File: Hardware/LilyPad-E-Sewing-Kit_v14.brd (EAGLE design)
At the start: 133.1 x 52.3 mm, 91 parts

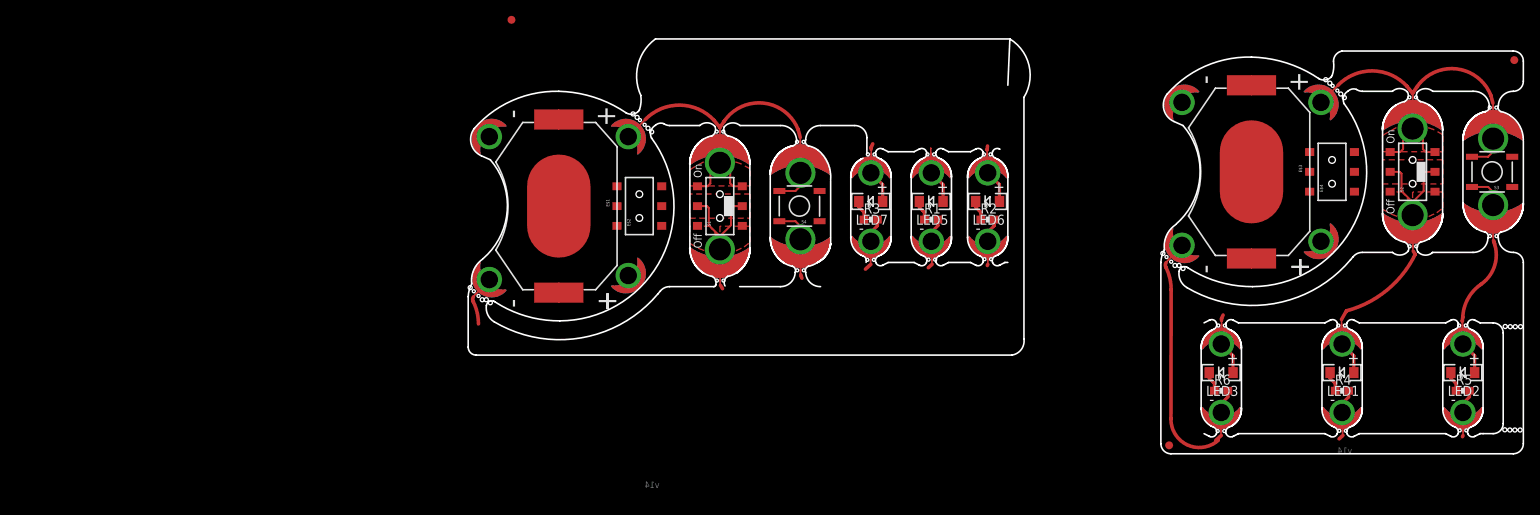
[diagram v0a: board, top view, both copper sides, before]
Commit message: Updated board file
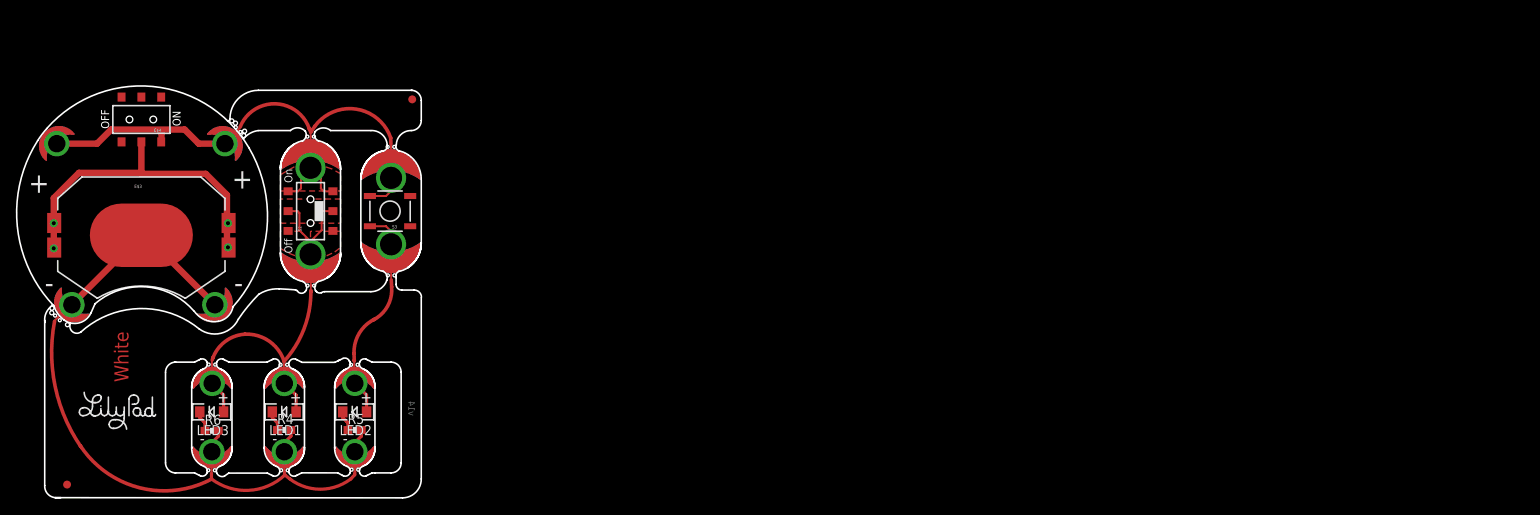
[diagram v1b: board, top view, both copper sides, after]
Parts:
- removed BUTTON-1, BUTTONS1, SLIDEOFF1, SLIDEON1: SEWTAP8, LilyPad-Wearables:PETAL-MEDIUM-2SIDE
- removed E$1: (no value), SparkFun-Electromechanical:BATTCON_20MM_4LEGS
- removed E$2: (no value), SparkFun-Electromechanical:AYZ0202
- removed JP4, JP6: LOGO-SFESK, SparkFun-Aesthetics:SFE-LOGO-FLAME
- removed JP5: FIDUCIAL1X2, SparkFun:FIDUCIAL-1X2
- removed LED+5, LED+6, LED+7, LED-5, LED-6, LED-7, U$34, U$35, U$36, U$37: SEWTAP6, LilyPad-Wearables:PETAL-SMALL-2SIDE
- removed LED5, LED6, LED7: White, SparkFun-3-2-07:LED-1206
- removed LOGO10, LOGO11, LOGO14, LOGO8, LOGO9: LOGO-LPL, LilyPad-Wearables:LOGO-L
- removed R1, R2, R3: 100, SparkFun:0603-RES
- removed S1: AYZ0202, SparkFun:AYZ0202
- removed S4: (no value), SparkFun:TACTILE_SWITCH_SMD
- removed U$18, U$43: OSHW-LOGOS, SparkFun-Aesthetics:OSHW-LOGO-S
- removed U$22, U$23, U$24, U$27, U$28, U$29, U$30, U$31, U$32, U$33, U$39, U$41: MOUSE-BITE-12_HOLES, Testing:MOUST-BITE-1-(2_HOLES)
- removed U$38: LOGO-LPLP, LilyPad-Wearables:LOGO-LILYPAD
- added E$5: (no value), LilyPad-Wearables:LOGO-LILYPAD
- E$3: device SparkFun-Electromechanical:BATTCON_20MM_4LEGS -> SparkFun-Electromechanical:BATTCON_20MM_4LEGS_OVERPASTE
- R4, R5, R6: value 100 -> 180
- moved U$12 159.5 mm to (1.45, 44.7), turned to 223 degrees
- moved E$4 150.3 mm to (12.1, 47.8), turned to 180 degrees
- moved U$15 143.9 mm to (12.1, 37.0), turned to 0 degrees
- moved U$11 142.3 mm to (3.35, 24.4), turned to 317 degrees
- moved U$17 140.4 mm to (1.52, 22.7), turned to 45 degrees
- moved E$3 140.3 mm to (12.1, 33.1), turned to 0 degrees
- moved LED+2 139.9 mm to (39.0, 14.5)
- moved LED-2 139.9 mm to (39.0, 5.84)
- moved U$5 139.9 mm to (39.0, 3.58)
- moved LED2 139.9 mm to (39.0, 10.9)
- moved R5 139.9 mm to (39.0, 8.59)
- moved U$2 139.9 mm to (39.0, 16.8)
- moved LOGO5 139.8 mm to (39.1, 9.80)
- moved BUTTON-2 139.1 mm to (43.6, 40.1)
- moved BUTTONS2 139.1 mm to (43.6, 32.3)
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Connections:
- removed net BUTTON1: BUTTONS1.1, S4.2, U$31.P$1
- removed net N$1: LED5.C, R1.1
- removed net N$2: LED6.C, R2.1
- removed net N$3: LED7.C, R3.1
- removed net S$1: LED+7.1, LED7.A, U$22.P$1
- removed net S$10: LED+6.1, LED6.A, U$23.P$1
- removed net S$11: LED+5.1, LED5.A, U$24.P$1
- removed net S$3: LED-6.1, R2.2, U$28.P$1
- removed net S$4: LED-5.1, R1.2, U$29.P$1
- removed net S$9: U$34.1, U$36.1, U$41.P$1
- removed net SINK3: S1.4
- removed net SINK4: S1.1
- removed net SWITCH1: S1.2, S1.5, SLIDEOFF1.1, U$32.P$1
- removed net VCC1: BUTTON-1.1, S1.3, S1.6, S4.4, SLIDEON1.1, U$30.P$1, U$33.P$1, U$35.1, U$37.1, U$39.P$1
- new net S$16: LED+2.1, LED2.A
- new net S$25: U$2.P$1
- new net S$26: LED+1.1, LED1.A, U$3.P$1
- net BUTTON2: no longer LED+2.1, LED2.A, U$2.P$1
- net GND2: no longer U$17.P$1
- net S$2: now also U$14.1; no longer LED-7.1, R3.2, U$27.P$1
- net S$6: no longer U$6.P$1
- net S$8: no longer U$1.P$1
- net SWITCH2: no longer LED+1.1, LED1.A, U$3.P$1
- net VCC2: no longer U$12.1, U$14.1, U$16.P$1
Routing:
- net VCC1: track 47.5 -> 0.00 mm
- net SWITCH2: track 38.0 -> 17.7 mm
- net S$29: track 0.00 -> 19.2 mm
- net S$2: track 6.98 -> 25.6 mm
- net BUTTON2: track 27.5 -> 9.03 mm
- net SWITCH1: track 18.1 -> 0.00 mm
- net S$18: track 0.00 -> 17.1 mm
- net S$28: track 0.00 -> 16.1 mm
- net S$4: track 6.73 -> 22.8 mm
- net VCC2: track 47.5 -> 34.8 mm
- net S$23: track 0.00 -> 11.3 mm
- net S$10: track 7.63 -> 18.6 mm, vias 0 -> 2
- net BUTTON1: track 9.75 -> 0.00 mm
- net S$19: track 0.00 -> 9.63 mm
- net S$25: track 0.00 -> 8.73 mm
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- removed copper zone on layer 1, net GND1
- removed copper zone on layer 1, net SINK3
- removed copper zone on layer 1, net SINK4
- removed copper zone on layer 1, net VCC1
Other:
- board size 133.1 x 52.3 mm -> 51.1 x 52 mm
- board text added: "OFF"
- board text added: "ON"
- board text added: "White"
- board text removed: "Coin Cell Battery Holder"
- board text removed: "E-sewing Kit"
